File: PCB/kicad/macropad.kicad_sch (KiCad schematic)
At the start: 77 parts, among them J1 OLED_128x32, J2 4P4C, SW1 RESET_Push, SW2 RotaryEncoder_Switch, SW3 RotaryEncoder_Switch, SW4 RotaryEncoder_Switch, SW5 Soft_Push, SW6 Soft_Push, SW7 Soft_Push, U1 5-Way Nav, U2 NOT Gate, U3 ON/OFF

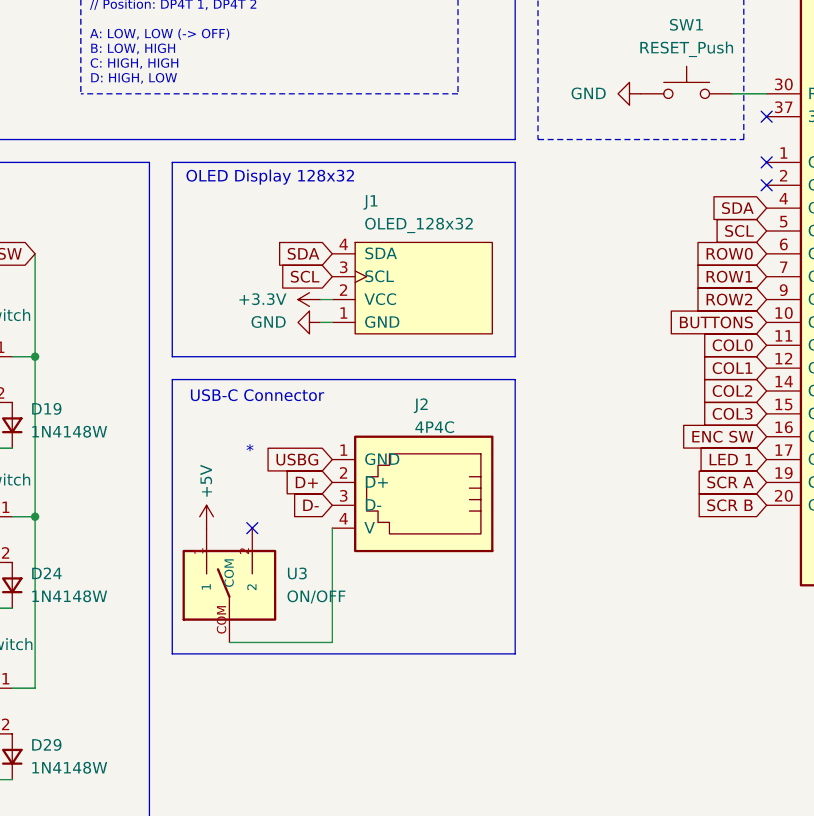
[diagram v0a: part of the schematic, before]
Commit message: Routed PCB
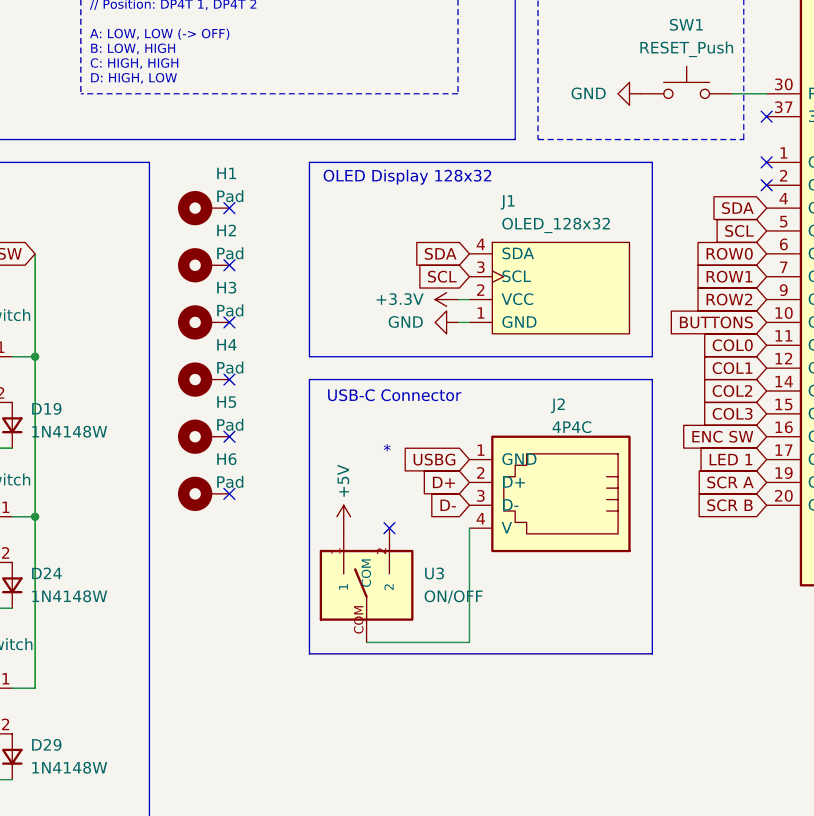
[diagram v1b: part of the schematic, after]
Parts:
- added H1, H2, H3, H4, H5, H6: Pad, MountingHole:MountingHole_2.2mm_M2_Pad, symbol Mechanical:MountingHole_Pad
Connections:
- no-connect marks 14 -> 20
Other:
- moved on the sheet: J1, J2, U3
